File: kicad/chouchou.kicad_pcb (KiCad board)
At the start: 2 copper layers, 212.4 x 114.4 mm, 41 parts

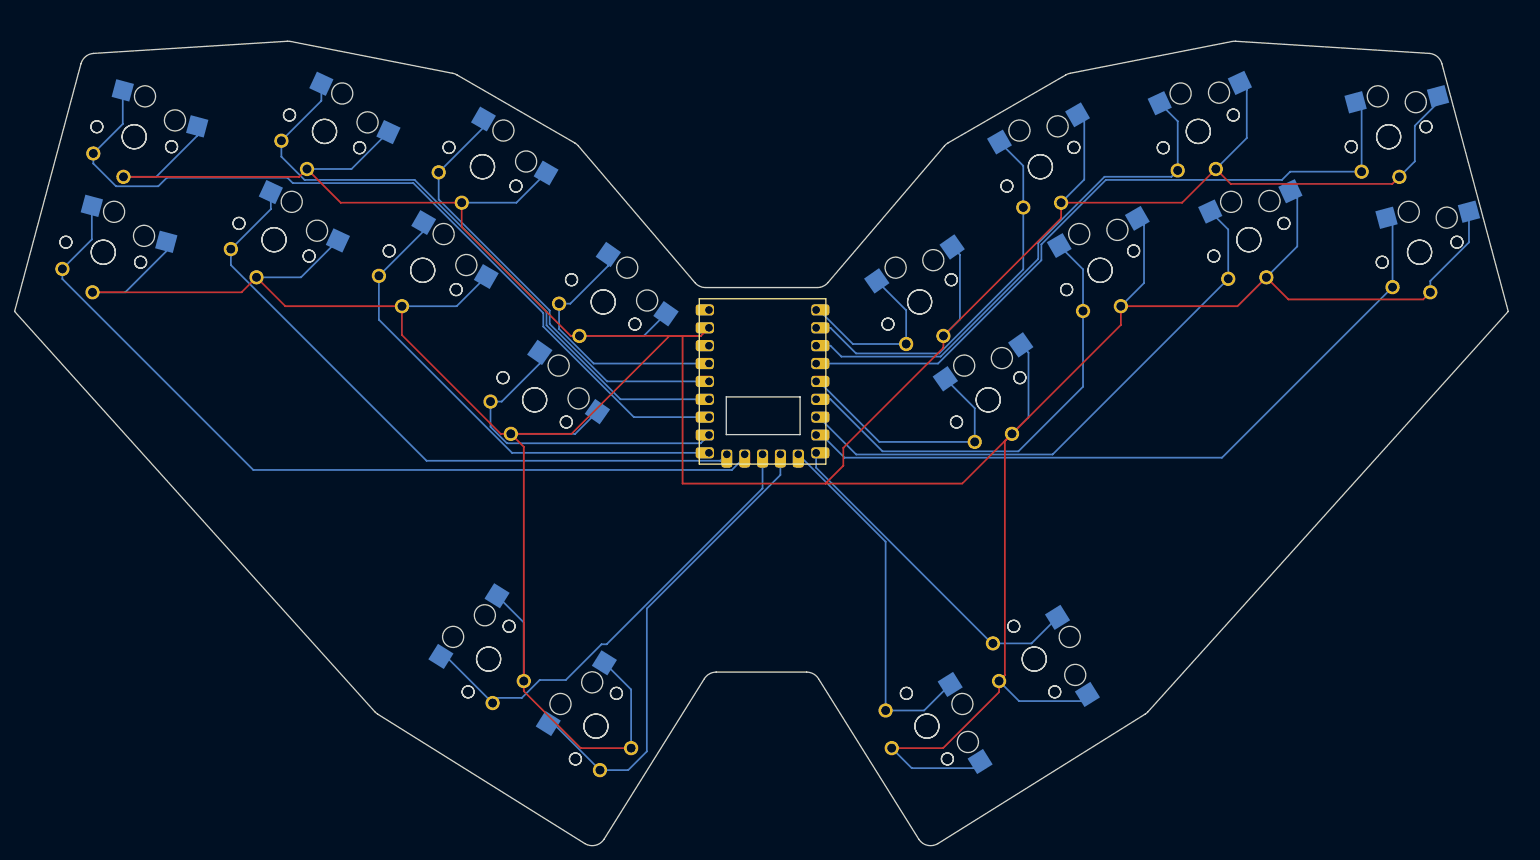
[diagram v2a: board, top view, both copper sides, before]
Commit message: Add images
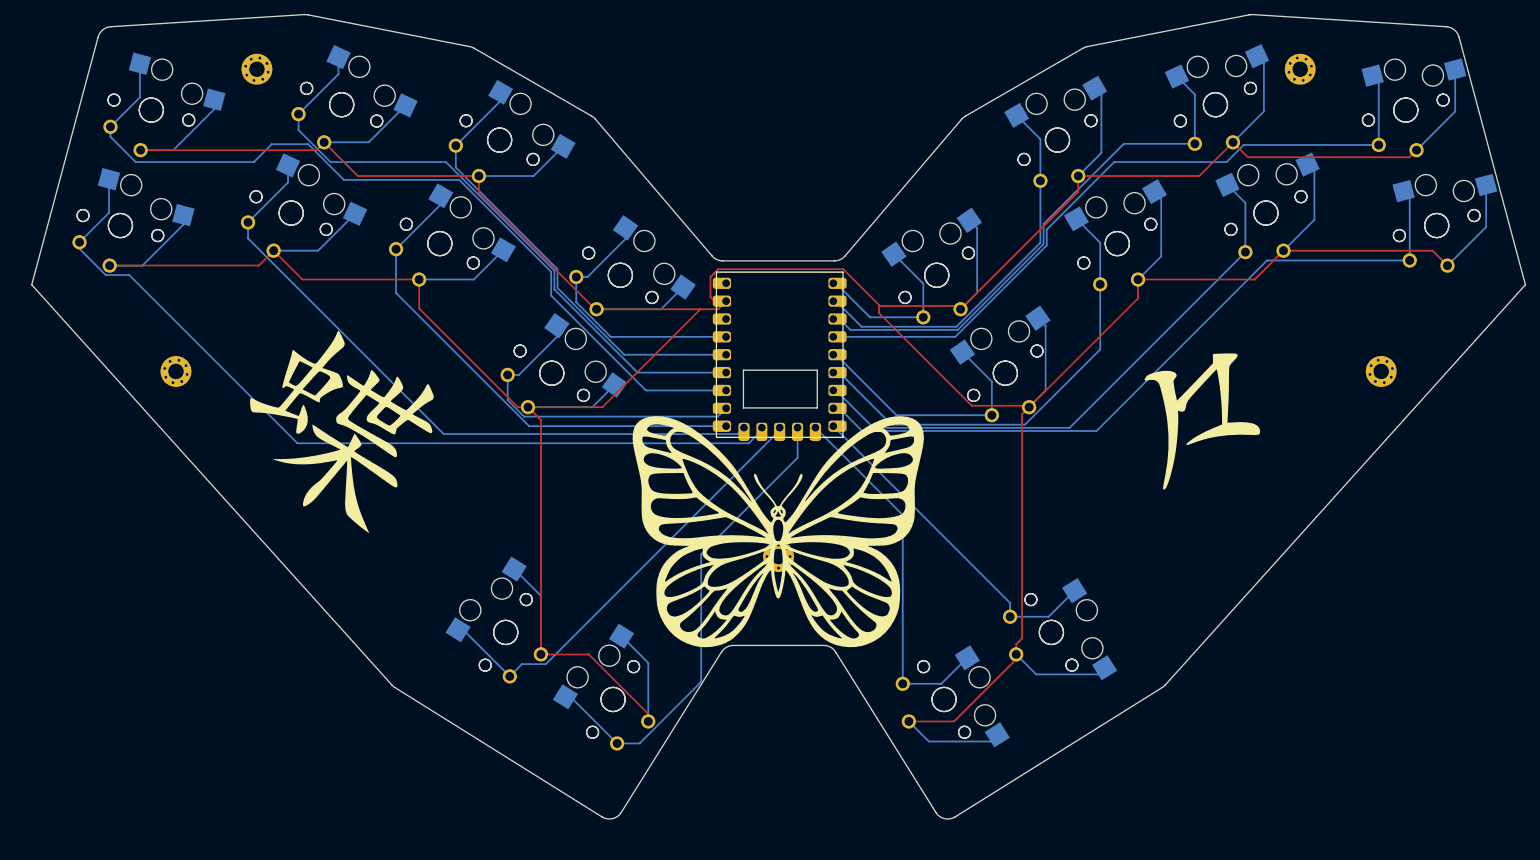
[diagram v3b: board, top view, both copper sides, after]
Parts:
- added ?: LOGO, images:蝶, F.Cu at (91.7, 98.5)
- added ?: LOGO, images:々, F.Cu at (213.7, 95.9)
- added G***: LOGO, images:butterfly, F.Cu at (153.3, 113.5)
- added _1: , MountingHole_2.2mm_M2_Pad_Via, F.Cu at (79.2, 47.8)
- added _2: , MountingHole_2.2mm_M2_Pad_Via, F.Cu at (67.7, 90.7)
- added _3: , MountingHole_2.2mm_M2_Pad_Via, F.Cu at (227.5, 47.8)
- added _4: , MountingHole_2.2mm_M2_Pad_Via, F.Cu at (239.1, 90.7)
- added _5: , MountingHole_2.2mm_M2_Pad_Via, F.Cu at (153.4, 117.1)
- moved S11 4.51 mm to (247.0, 70.0)
- moved S31 4.51 mm to (247.0, 70.0)
- moved S20 4.51 mm to (176.9, 137.4)
- moved S40 4.51 mm to (176.9, 137.4)
- moved S27 4.51 mm to (121.1, 91.0)
- moved S7 4.51 mm to (121.1, 91.0)
- moved S12 4.51 mm to (242.6, 53.6)
- moved S16 4.51 mm to (193.0, 57.8)
- moved S2 4.51 mm to (64.2, 53.6)
- moved S22 4.51 mm to (64.2, 53.6)
- moved S26 4.51 mm to (113.7, 57.8)
- moved S32 4.51 mm to (242.6, 53.6)
- moved S36 4.51 mm to (193.0, 57.8)
- moved S6 4.51 mm to (113.7, 57.8)
- moved S10 4.51 mm to (129.8, 137.4)
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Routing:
- net GND: track 840.4 -> 808.7 mm
- net GP11: track 66.0 -> 63.4 mm
- net GP26: track 116.8 -> 118.7 mm
- net GP5: track 66.3 -> 65.4 mm

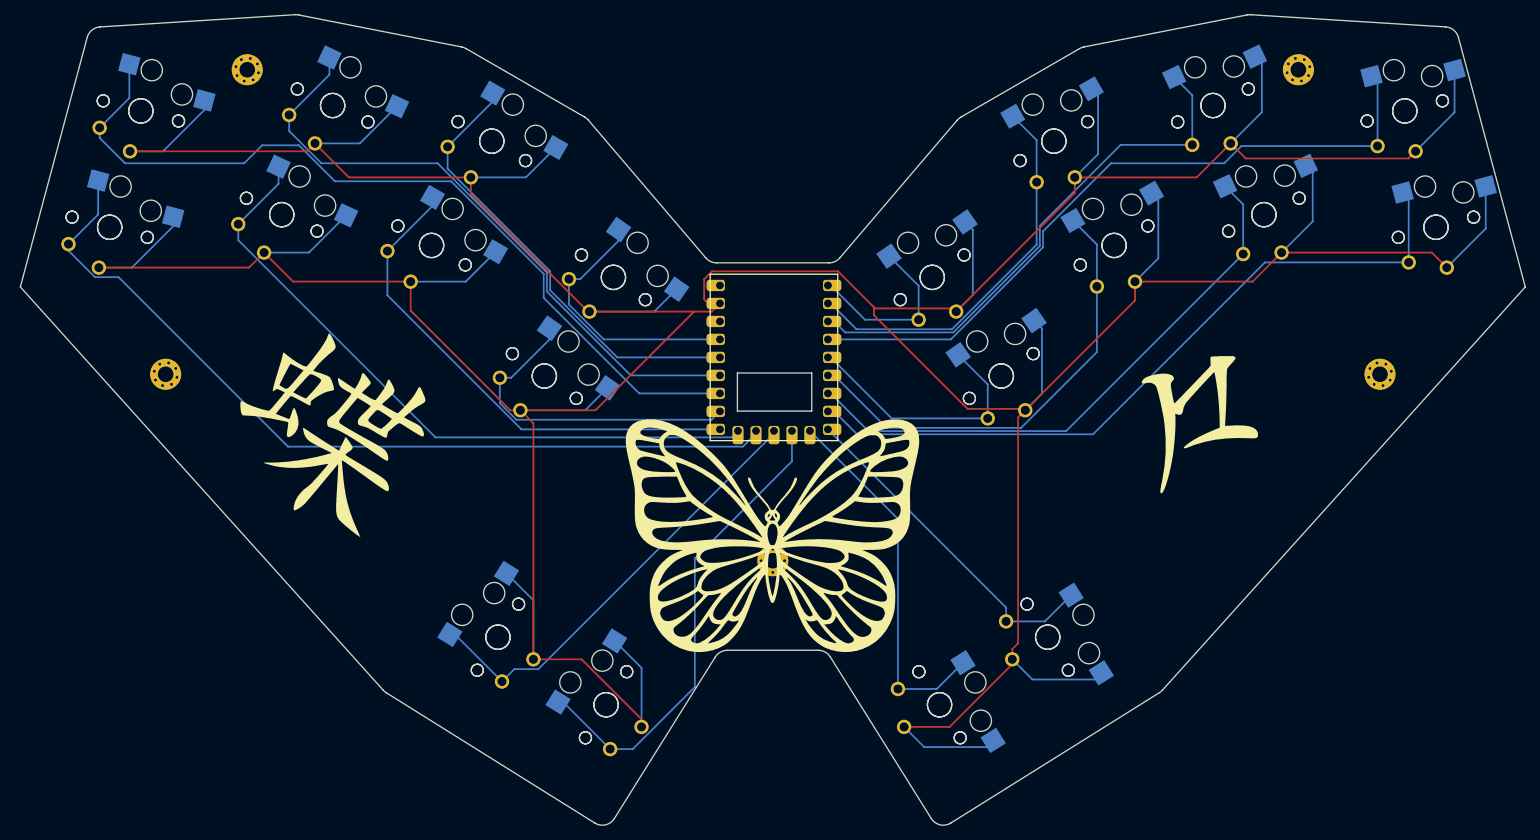
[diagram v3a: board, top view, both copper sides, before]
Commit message: Add ordered files
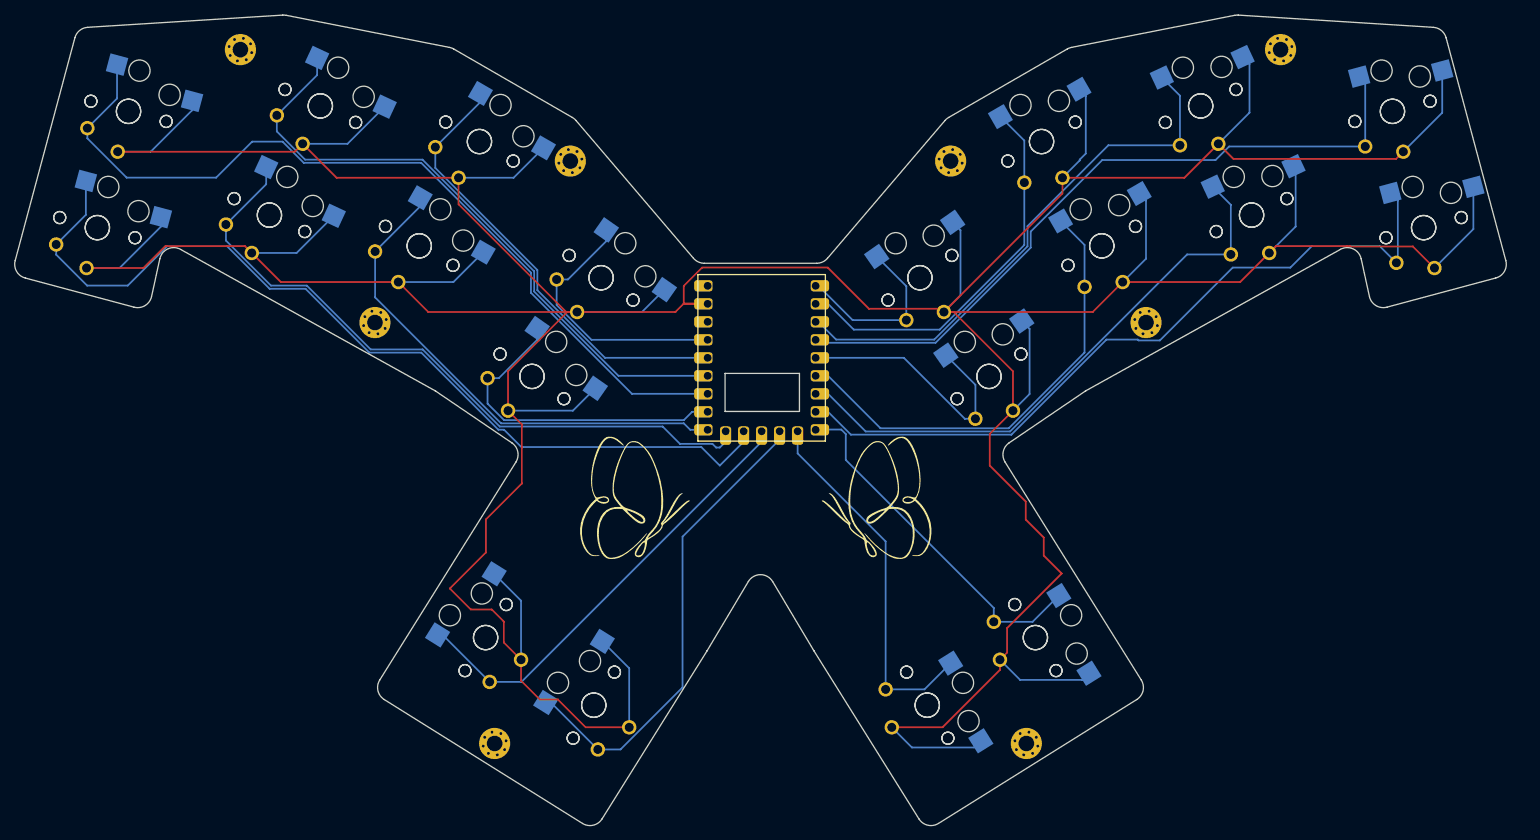
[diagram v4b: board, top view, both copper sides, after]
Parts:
- removed the ? at (91.7, 98.5)
- removed the ? at (213.7, 95.9)
- removed G***: LOGO, images:butterfly
- added ?: LOGO, images:butterfly_right, F.Cu at (168.7, 108.7)
- added ?: LOGO, images:butterfly_left, F.Cu at (133.2, 108.7)
- added _6: , MountingHole_2.2mm_M2_Pad_Via, F.Cu at (178.5, 60.6)
- added _7: , MountingHole_2.2mm_M2_Pad_Via, F.Cu at (114.1, 142.9)
- added _8: , MountingHole_2.2mm_M2_Pad_Via, F.Cu at (189.1, 142.9)
- moved _2 163.9 mm to (225.0, 44.9), turned to 15 degrees
- moved _3 135.1 mm to (97.2, 83.4), turned to -30 degrees
- moved _5 63.2 mm to (124.8, 60.6), turned to -35 degrees
- moved _4 33.8 mm to (206.0, 83.4), turned to 30 degrees
- moved _1 3.00 mm to (78.2, 44.9)
- moved RP2040Zero1 1.74 mm to (141.6, 101.1)
- moved S11 1.74 mm to (245.2, 70.0)
- moved S12 1.74 mm to (240.8, 53.6)
- moved S14 1.74 mm to (213.7, 52.9)
- moved S17 1.74 mm to (183.9, 91.0)
- moved S18 1.74 mm to (174.1, 77.1)
- moved S19 1.74 mm to (190.4, 127.9)
- moved S27 1.74 mm to (119.4, 91.0)
- moved S28 1.74 mm to (129.1, 77.1)
- moved S29 1.74 mm to (112.8, 127.9)
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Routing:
- net GND: track 808.7 -> 819.8 mm
- net GP12: track 121.3 -> 129.0 mm
- net GP7: track 103.6 -> 105.8 mm
- net GP13: track 95.2 -> 97.2 mm
- net GP26: track 118.7 -> 120.5 mm
- net GP2: track 75.3 -> 76.1 mm
- net GP11: track 63.4 -> 64.0 mm
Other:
- board size 212.4 x 114.4 mm -> 210.5 x 114.4 mm

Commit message: Connect pcb
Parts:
- removed ?: LOGO, images:butterfly_right
- removed ?: LOGO, images:butterfly_left
- added RP2040Zero2: , RP2040-Zero, F.Cu at (158.3, 78.8)
- added S41, S58: , PG1350, F.Cu at (227.4, 67.1)
- added S42, S59: , PG1350, F.Cu at (227.4, 50.1)
- added S43, S60: , PG1350, F.Cu at (227.4, 33.1)
- added S44, S61: , PG1350, F.Cu at (209.2, 72.7)
- added S45, S62: , PG1350, F.Cu at (208.3, 55.7)
- added S46, S63: , PG1350, F.Cu at (207.4, 38.7)
- added S47, S64: , PG1350, F.Cu at (191.4, 77.0)
- added S48, S65: , PG1350, F.Cu at (190.5, 60.0)
- added S49, S66: , PG1350, F.Cu at (189.6, 43.1)
- added S50, S67: , PG1350, F.Cu at (203.4, 100.2)
- added S51, S68: , PG1350, F.Cu at (183.4, 105.0)
- added S52: , PG1350, F.Cu at (264.8, 80.0)
- added S53: , PG1350, F.Cu at (266.3, 63.1)
- added S54: , PG1350, F.Cu at (267.8, 46.1)
- added S55: , PG1350, F.Cu at (245.4, 72.7)
- added S56: , PG1350, F.Cu at (245.4, 55.7)
- added S57: , PG1350, F.Cu at (245.4, 38.7)
- added TRRS1: TRRS-PJ-320A-dual, TRRS-PJ-320A-dual, F.Cu at (138.0, 86.1)
- added TRRS2: TRRS-PJ-320A-dual, TRRS-PJ-320A-dual, F.Cu at (156.8, 81.6)
- moved S19 174.4 mm to (28.5, 63.1), turned to -175 degrees
- moved S20 174.0 mm to (27.0, 46.1), turned to -175 degrees
- moved _2 161.2 mm to (67.4, 79.1), turned to 0 degrees
- moved S11 159.3 mm to (86.5, 55.7), turned to -3 degrees
- moved S12 154.1 mm to (87.4, 38.7), turned to -3 degrees
- moved _7 152.9 mm to (214.0, 27.2), turned to 3 degrees
- moved S18 144.1 mm to (30.0, 80.0), turned to -175 degrees
- moved S31 141.3 mm to (104.3, 60.0), turned to 177 degrees
- moved _5 136.7 mm to (258.8, 33.8), turned to -5 degrees
- moved S32 136.0 mm to (105.2, 43.1), turned to 177 degrees
- moved S33 133.4 mm to (91.4, 100.2), turned to -96 degrees
- moved S40 121.2 mm to (245.4, 38.7), turned to 0 degrees
- moved S13 117.8 mm to (103.4, 77.0), turned to -3 degrees
- moved S34 114.9 mm to (111.4, 105.0), turned to -111 degrees
- moved _4 111.2 mm to (98.8, 112.8), turned to 69 degrees
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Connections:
- RP2040Zero1 pad 10: GP9 -> matrix_outer_bottom
- RP2040Zero1 pad 11: GP10 -> matrix_pinky_middle
- RP2040Zero1 pad 12: GP11 -> matrix_ring_middle
- RP2040Zero1 pad 13: GP12 -> matrix_middle_middle
- RP2040Zero1 pad 14: GP13 -> matrix_index_middle
- RP2040Zero1 pad 15: GP14 -> matrix_outer_middle
- RP2040Zero1 pad 16: GP15 -> matrix_pinky_top
- RP2040Zero1 pad 17: GP26 -> matrix_ring_top
- RP2040Zero1 pad 18: GP27 -> matrix_middle_top
- RP2040Zero1 pad 2: GP1 -> SCL
- RP2040Zero1 pad 22: GP28 -> matrix_index_top
- RP2040Zero1 pad 23: GP29 -> matrix_outer_top
- RP2040Zero1 pad 4: GP3 -> thumbs_outer_cluster
- RP2040Zero1 pad 5: GP4 -> thumbs_inner_cluster
- RP2040Zero1 pad 6: GP5 -> matrix_pinky_bottom
- RP2040Zero1 pad 7: GP6 -> matrix_ring_bottom
- RP2040Zero1 pad 8: GP7 -> matrix_middle_bottom
- RP2040Zero1 pad 9: GP8 -> matrix_index_bottom
- S1 pad 1: GP12 -> matrix_pinky_bottom
- S10 pad 1: GP10 -> matrix_index_bottom
- S11 pad 1: GP7 -> matrix_index_middle
- S12 pad 1: GP3 -> matrix_index_top
- S13 pad 1: GP6 -> matrix_outer_bottom
- S14 pad 1: GP2 -> matrix_outer_middle
- S15 pad 1: GP5 -> matrix_outer_top
- S16 pad 1: GP1 -> thumbs_inner_cluster
- S17 pad 1: GP4 -> thumbs_outer_cluster
- S18 pad 1: GP0 -> matrix_pinky_bottom
- S19 pad 1: GP8 -> matrix_pinky_middle
- S2 pad 1: GP26 -> matrix_pinky_middle
- S20 pad 1: GP9 -> matrix_pinky_top
- S21 pad 1: GP12 -> matrix_ring_bottom
- S22 pad 1: GP26 -> matrix_ring_middle
- S23 pad 1: GP13 -> matrix_ring_top
- S24 pad 1: GP27 -> matrix_middle_bottom
- S25 pad 1: GP14 -> matrix_middle_middle
- S26 pad 1: GP28 -> matrix_middle_top
- S27 pad 1: GP15 -> matrix_index_bottom
- S28 pad 1: GP29 -> matrix_index_middle
- S29 pad 1: GP11 -> matrix_index_top
- S3 pad 1: GP13 -> matrix_pinky_top
- S30 pad 1: GP10 -> matrix_outer_bottom
- S31 pad 1: GP7 -> matrix_outer_middle
- S32 pad 1: GP3 -> matrix_outer_top
- S33 pad 1: GP6 -> thumbs_inner_cluster
- S34 pad 1: GP2 -> thumbs_outer_cluster
- S35 pad 1: GP5 -> mirror_matrix_pinky_bottom
- S35 pad 2: GND -> rGND
- S36 pad 1: GP1 -> mirror_matrix_pinky_middle
- S36 pad 2: GND -> rGND
- S37 pad 1: GP4 -> mirror_matrix_pinky_top
- S37 pad 2: GND -> rGND
- S38 pad 1: GP0 -> mirror_matrix_ring_bottom
- S38 pad 2: GND -> rGND
- S39 pad 1: GP8 -> mirror_matrix_ring_middle
- S39 pad 2: GND -> rGND
- S4 pad 1: GP27 -> matrix_ring_bottom
- S40 pad 1: GP9 -> mirror_matrix_ring_top
- S40 pad 2: GND -> rGND
- S5 pad 1: GP14 -> matrix_ring_middle
- S6 pad 1: GP28 -> matrix_ring_top
- S7 pad 1: GP15 -> matrix_middle_bottom
- S8 pad 1: GP29 -> matrix_middle_middle
- S9 pad 1: GP11 -> matrix_middle_top
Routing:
- net rGND: track 0.00 -> 522.7 mm
- net GND: track 819.8 -> 444.7 mm
- net matrix_pinky_bottom: track 0.00 -> 144.9 mm
- net matrix_pinky_top: track 0.00 -> 132.7 mm
- net matrix_pinky_middle: track 0.00 -> 132.1 mm
- net GP12: track 129.0 -> 0.00 mm
- net matrix_ring_bottom: track 0.00 -> 122.3 mm
- net GP26: track 120.5 -> 0.00 mm
- net mirror_matrix_pinky_middle: track 0.00 -> 115.4 mm
- net mirror_matrix_pinky_bottom: track 0.00 -> 114.1 mm
- net mirror_matrix_pinky_top: track 0.00 -> 111.4 mm
- net matrix_ring_middle: track 0.00 -> 108.9 mm
- net matrix_ring_top: track 0.00 -> 106.8 mm
- net GP7: track 105.8 -> 0.00 mm
- net GP3: track 100.8 -> 0.00 mm
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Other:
- board size 210.5 x 114.4 mm -> 262.1 x 95.9 mm
